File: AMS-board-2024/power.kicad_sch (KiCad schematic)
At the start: 61 parts, among them Q109 DMT6007LFGQ, Q110 BSS308PE, Q111 2N7002K-AU, Q112 2N7002K-AU, Q113 DMT6007LFGQ, Q114 2N7002K-AU, U18 UCC12040, U19 AP74700QW6-7, U20 VOMA617A, U21 LM5060, U22 LMR33620APCQRNXRQ1

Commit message: およそ回路図完成
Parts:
- D123, D124: footprint (none) -> LED_SMD:LED_0603_1608Metric
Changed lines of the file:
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@@
       (effects (font (size 1.27 1.27)) (justify right))
     )
-    (property "Footprint" "" (at 63.5 44.45 0)
+    (property "Footprint" "LED_SMD:LED_0603_1608Metric" (at 63.5 44.45 0)
       (effects (font (size 1.27 1.27)) hide)
     )
@@
       (effects (font (size 1.27 1.27)) (justify left))
     )
-    (property "Footprint" "" (at 50.8 44.45 0)
-      (effects (font (size 1.27 1.27)) hide)
-    )
+    (property "Footprint" "LED_SMD:LED_0603_1608Metric" (at 50.8 44.45 0)
+      (effects (font (size 1.27 1.27)) hide)
+    )

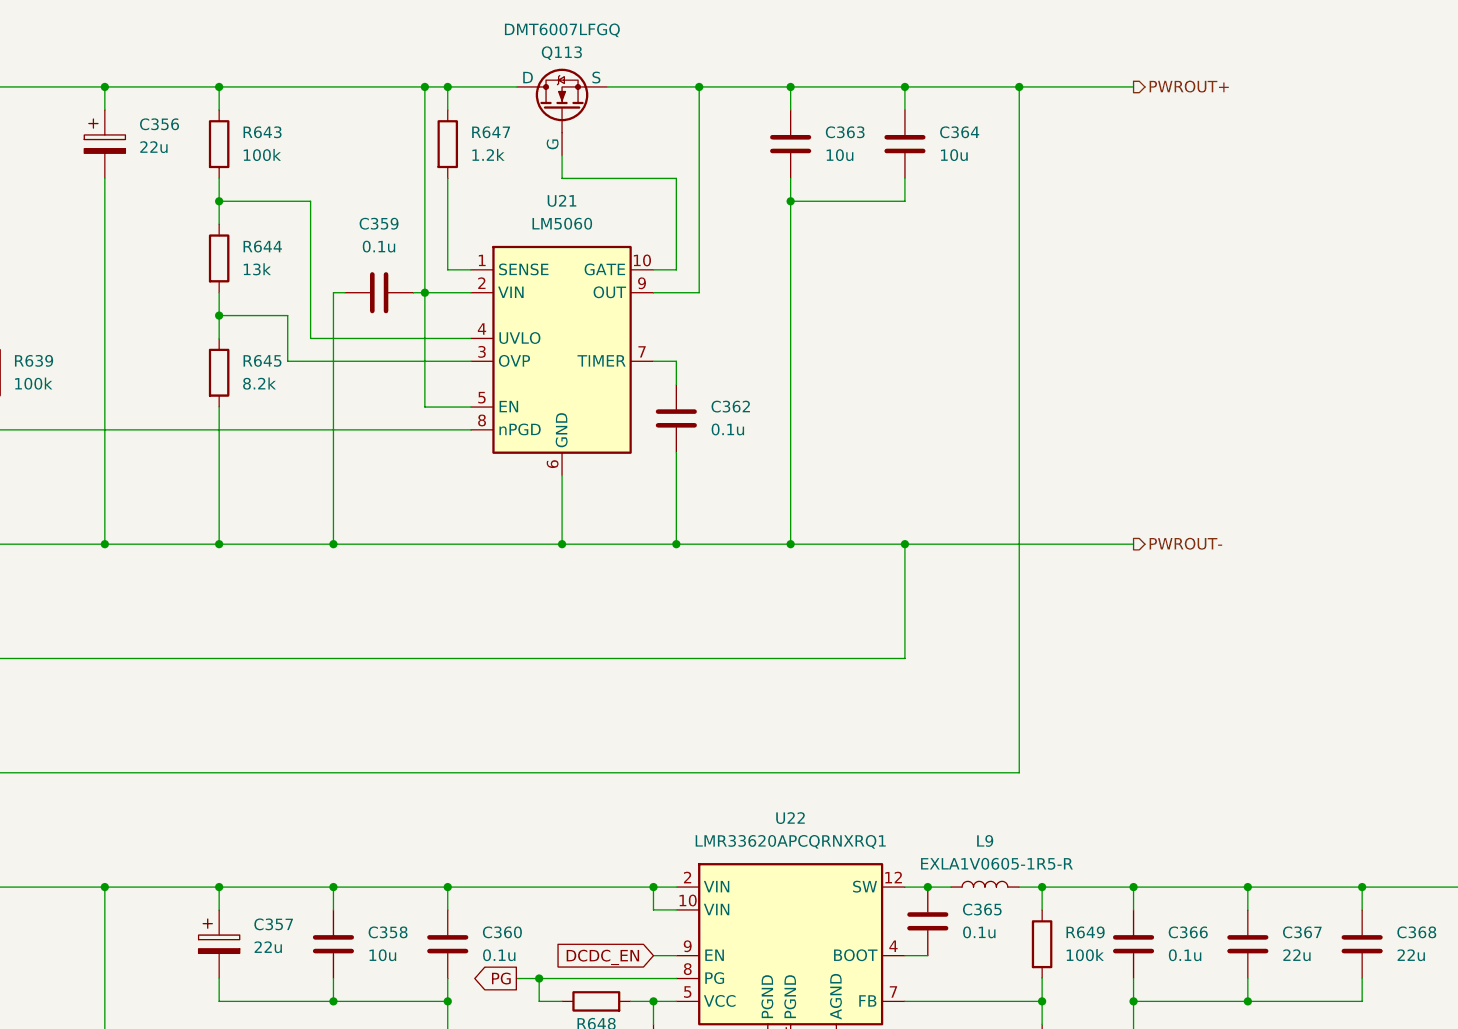
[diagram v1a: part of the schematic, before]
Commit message: 設定値記載
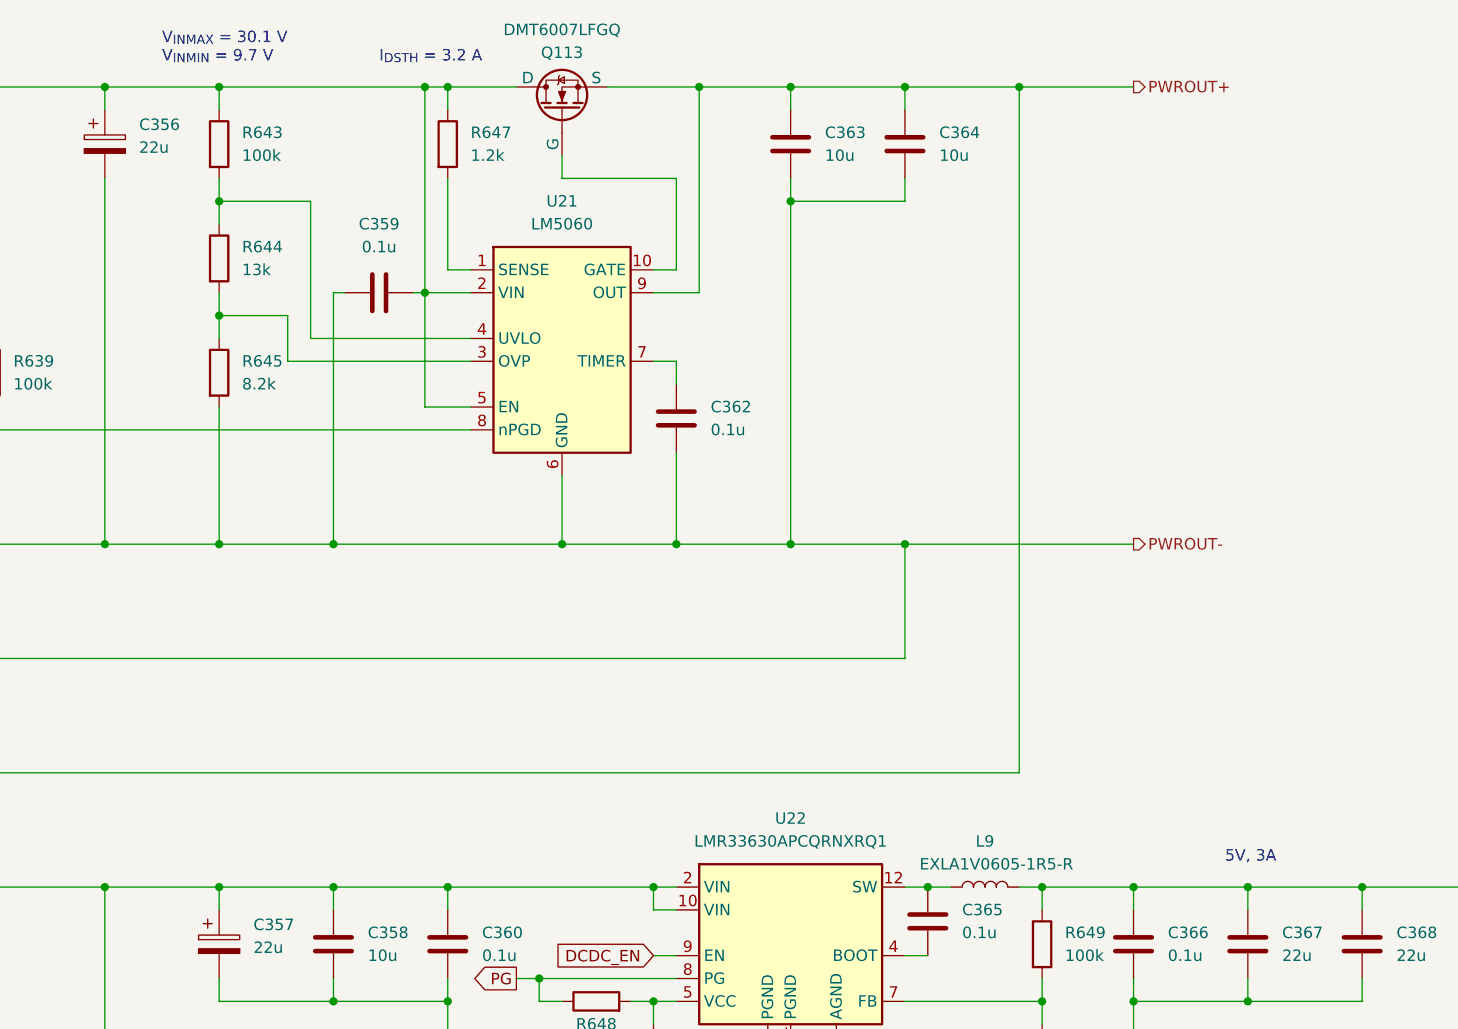
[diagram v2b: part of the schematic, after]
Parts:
- U22: value LMR33620APCQRNXRQ1 -> LMR33630APCQRNXRQ1
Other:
- note added: "5V, 3A"
- note added: "I_{DSTH} = 3.2 A"
- note added: "V_{INMAX} = 30.1 V V_{INMIN} = 9.7 V"
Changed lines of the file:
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@@
     (stroke (width 0) (type default))
+  )
+  (text "V_{INMAX} = 30.1 V\nV_{INMIN} = 9.7 V" (at 196.85 35.56 0)
+    (effects (font (size 1.27 1.27)) (justify left bottom))
+  )
+  (text "I_{DSTH} = 3.2 A" (at 220.98 35.56 0)
+    (effects (font (size 1.27 1.27)) (justify left bottom))
+  )
+  (text "5V, 3A " (at 314.96 124.46 0)
+    (effects (font (size 1.27 1.27)) (justify left bottom))
   )
   (global_label "~{DCDC_EN}" (shape output) (at 175.26 76.2 180) (fields_autoplaced)
@@
       (effects (font (size 1.27 1.27)))
     )
-    (property "Value" "LMR33620APCQRNXRQ1" (at 266.7 121.92 0)
-      (effects (font (size 1.27 1.27)))
-    )
+    (property "Value" "LMR33630APCQRNXRQ1" (at 266.7 121.92 0)
+      (effects (font (size 1.27 1.27)))
+    )
